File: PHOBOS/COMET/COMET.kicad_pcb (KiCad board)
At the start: 4 copper layers, 63.5 x 25.4 mm, 73 parts, among them J2 M/D, J5 Power/Arm, J6 USB4056-03-A_REVA2, Q1 SISS67DN-T1-GE3, Q2 BSD840N, Q3 SISS67DN-T1-GE3, SW3 KMR211GLFS, U1 MPL3115A2, U2 LSM6DS3, U3 W25Q128JVSIQ, U4 NCP1117-3.3_SOT223, U5 RP2040, Y1 ABM8-272-T3

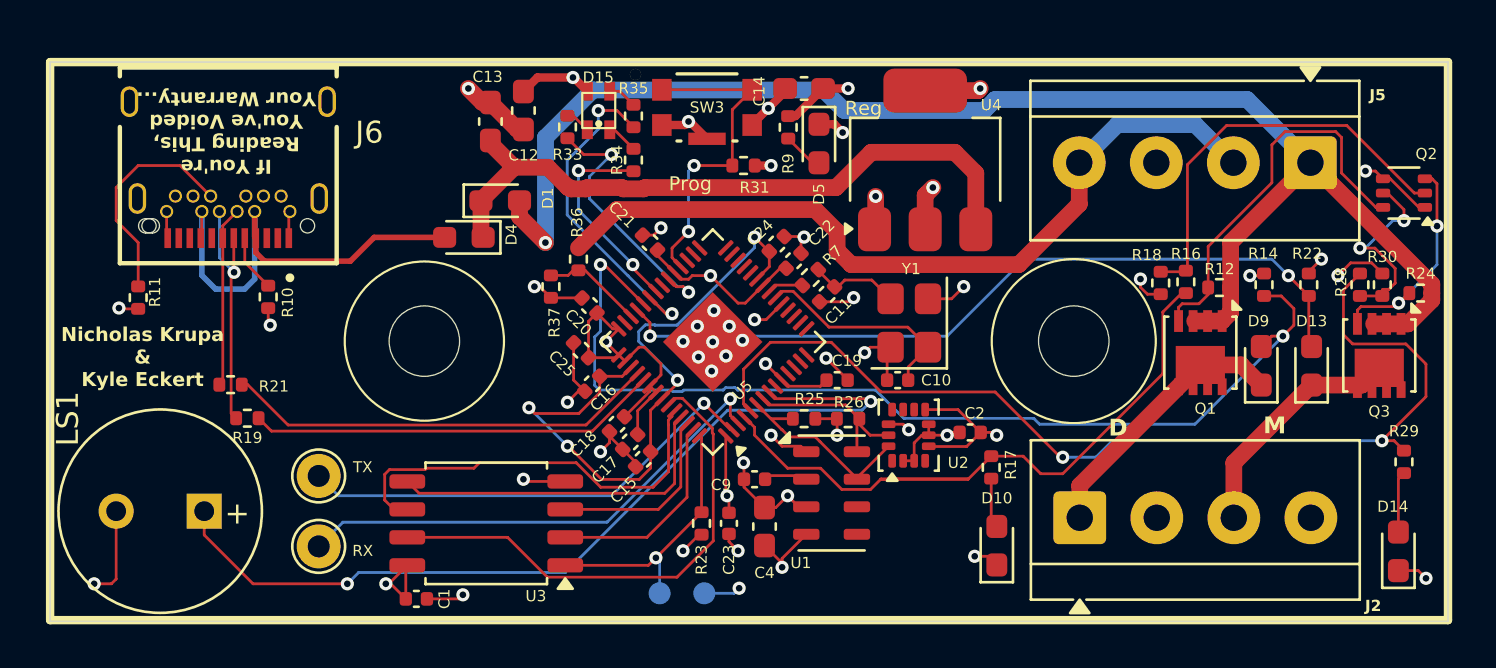
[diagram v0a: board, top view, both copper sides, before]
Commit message: unrouted, relocated, centering ensured. Dimensions added.
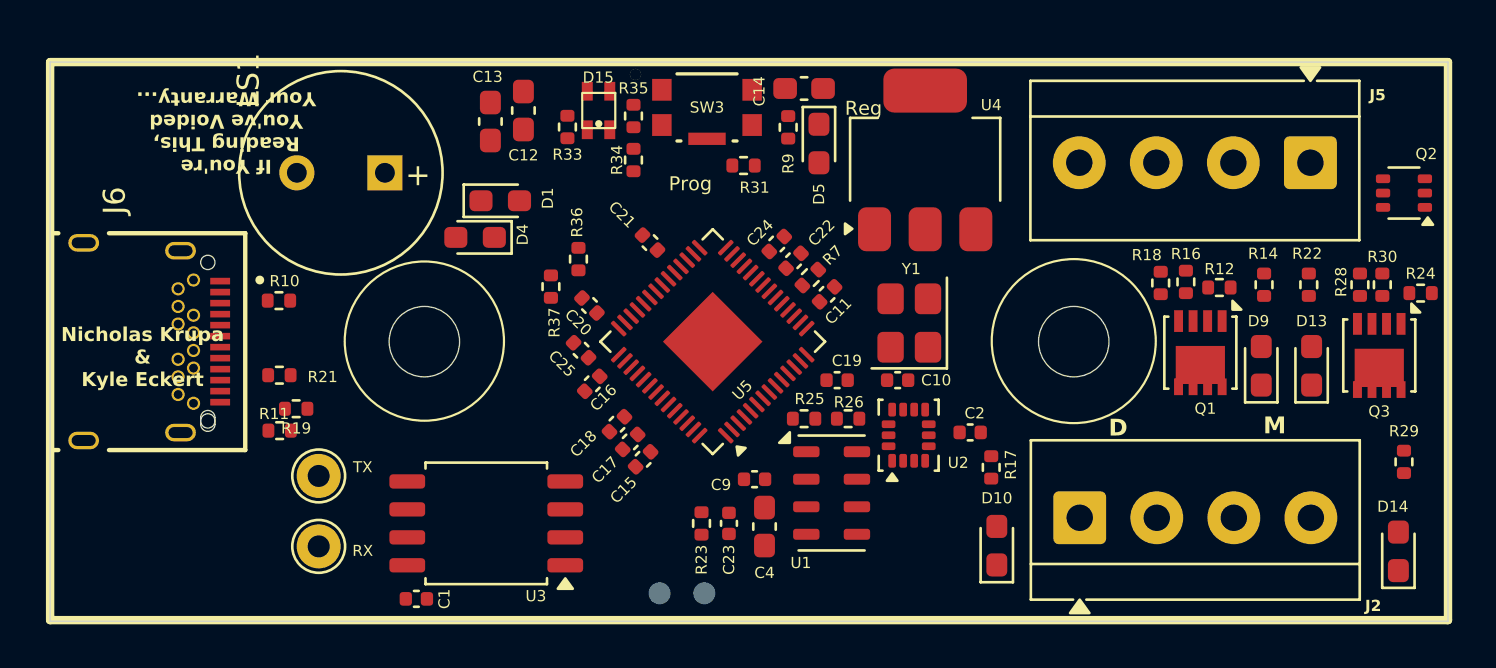
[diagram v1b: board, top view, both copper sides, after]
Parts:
- moved LS1 17.4 mm to (82.5, 65.9)
- moved J6 12.7 mm to (68.8, 73.6), turned to -90 degrees
- moved R11 8.82 mm to (77.7, 77.6), turned to 180 degrees
- moved R19 2.26 mm to (78.4, 76.6)
- moved R21 2.26 mm to (77.7, 75.1)
- moved R10 0.52 mm to (77.7, 71.7), turned to 0 degrees
- moved D4 0.51 mm to (86.6, 68.8)
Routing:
- net VMOS: track 66.4 -> 0.00 mm, vias 1 -> 0
- net GND: track 64.9 -> 0.00 mm, vias 39 -> 0
- net +3V3: track 62.7 -> 0.00 mm, vias 18 -> 0
- net /MOS_D: track 46.9 -> 0.00 mm, vias 2 -> 0
- net /MAIN_CONT: track 46.3 -> 0.00 mm, vias 2 -> 0
- net /Speaker: track 40.5 -> 0.00 mm, vias 2 -> 0
- net +BATT: track 36.5 -> 0.00 mm
- net /DROGUE_CONT: track 35.8 -> 0.00 mm, vias 2 -> 0
- net /MOS_M: track 31.6 -> 0.00 mm
- net V+: track 30.6 -> 0.00 mm
- net +1V1: track 30.3 -> 0.00 mm, vias 4 -> 0
- net /QSPI_SD3: track 23.1 -> 0.00 mm
- net /RX: track 22.8 -> 0.00 mm, vias 1 -> 0
- net /TX: track 21.9 -> 0.00 mm, vias 1 -> 0
- net VBUS: track 21.1 -> 0.00 mm
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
